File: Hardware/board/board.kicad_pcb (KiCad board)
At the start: 2 copper layers, 124 parts, among them J1 USB_C_Receptacle_USB2.0_16P, J2 Barrel_Jack_PTH, SW1 SKRPACE010, SW10 CPG151101D212, SW11 CPG151101D212, SW12 EC11E15244G1, SW13 EC11E15244G1, SW14 EC11E15244G1, SW15 EC11E15244G1, SW2 CPG151101D212, SW3 CPG151101D212, SW4 EC11E15244G1, SW5 CPG151101D212, SW6 CPG151101D212, SW7 CPG151101D212, SW8 CPG151101D212, SW9 EC11E15244G1, U1 MIC5219-3.3YM5, U10 WS2812B, U11 WS2812B, U12 WS2812B, U13 WS2812B, U14 WS2812B, U15 WS2812B, U16 WS2812B, U17 WS2812B, U18 WS2812B, U19 WS2812B, U2 MIC5219-3.3YM5, U20 WS2812B, U21 WS2812B, U22 WS2812B, U23 WS2812B, U24 WS2812B, U25 WS2812B, U26 WS2812B, U27 WS2812B, U28 WS2812B, U29 WS2812B, U3 STM32F407VETx, U30 WS2812B, U31 WS2812B, U32 WS2812B, U33 WS2812B, U34 WS2812B, U35 WS2812B, U36 WS2812B, U37 WS2812B, U38 WS2812B, U39 WS2812B, U4 PT4103B23F, U40 WS2812B, U41 WS2812B, U42 WS2812B, U43 WS2812B, U44 WS2812B, U45 WS2812B, U46 WS2812B, U47 WS2812B, U48 TPS562200DDCR, U49 TPS568215RNNR, U5 HC-FPC-0.5-40P-FH20, U50 CYA0630-4.7UH, U6 WS2812B, U7 WS2812B, U8 WS2812B, U9 WS2812B, X1 CSTNE8M00G550000R0

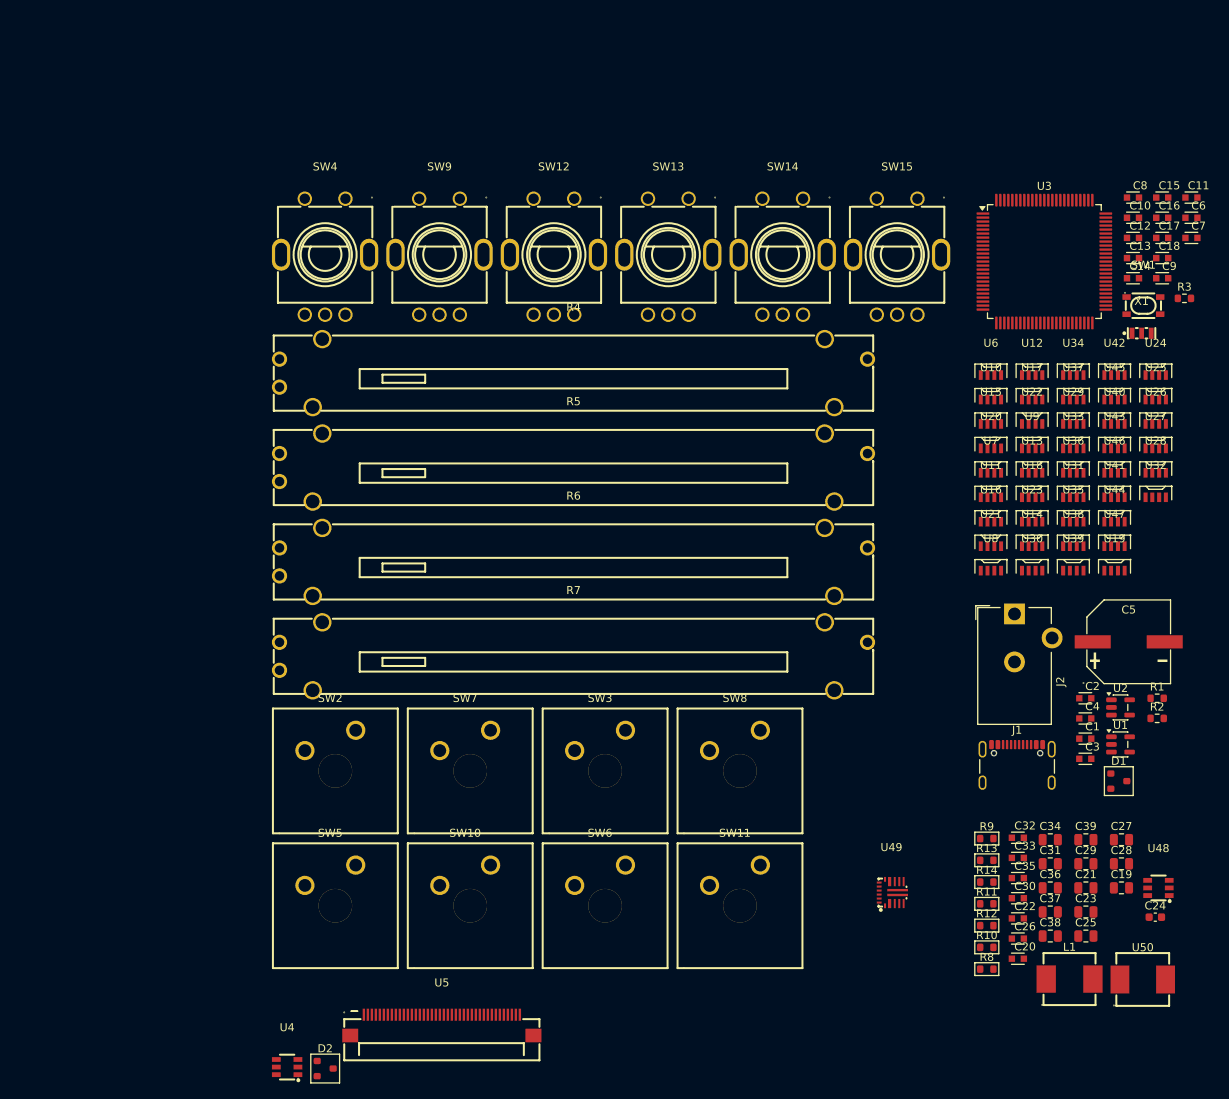
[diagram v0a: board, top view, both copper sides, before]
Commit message: sdadsa
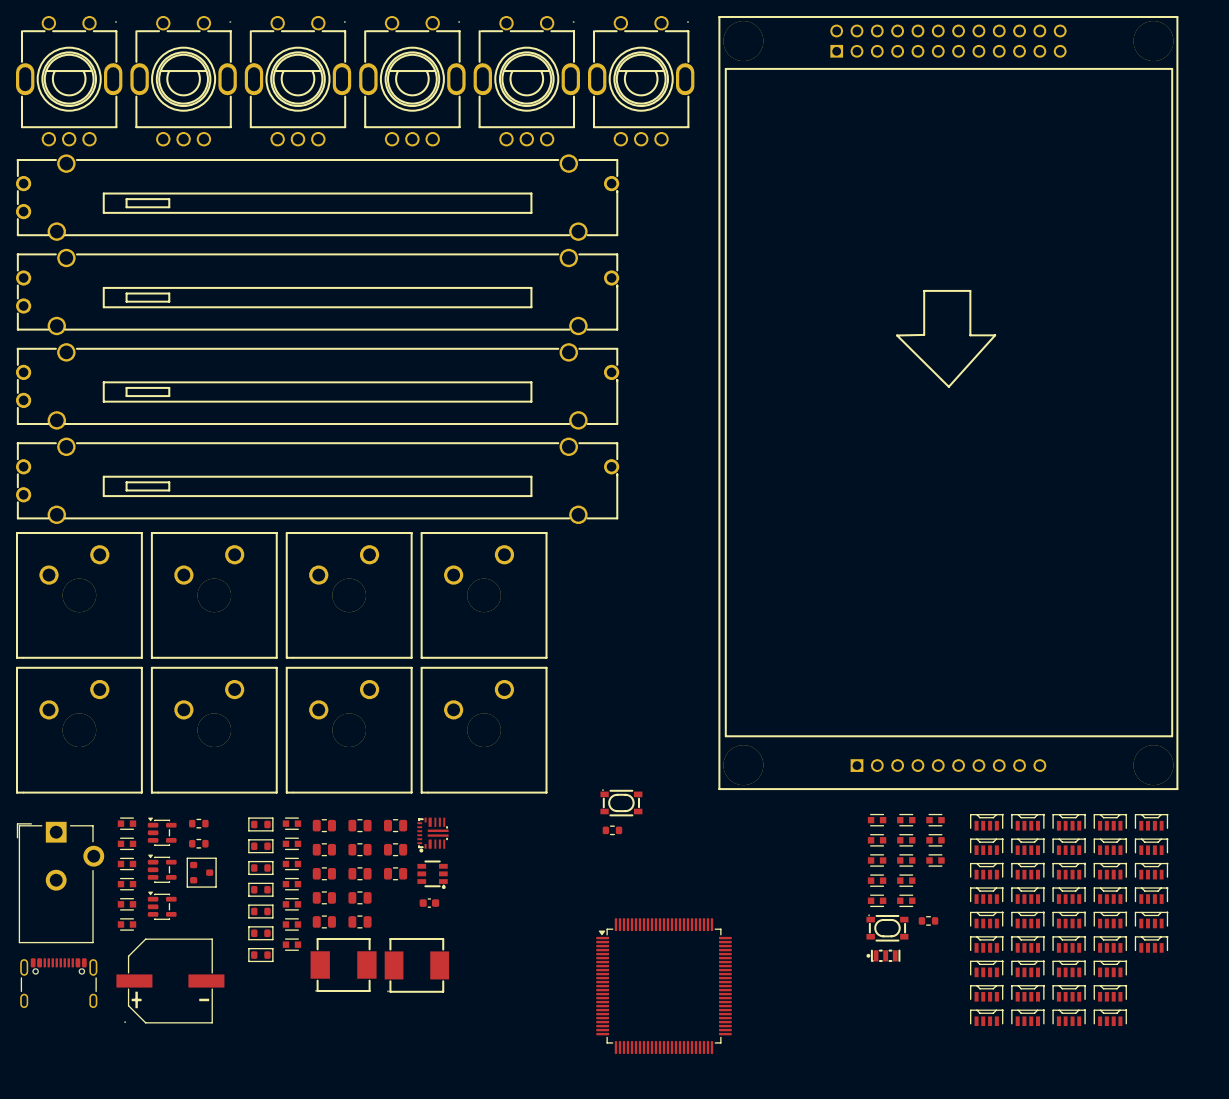
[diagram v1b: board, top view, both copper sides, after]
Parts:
- removed D2: PMEG4005CT, PCM_Package_TO_SOT_SMD_AKL:SOT-23
- removed U5: HC-FPC-0.5-40P-FH20, easyeda_imports:FPC-SMD_40P-P0.50_HC-FPC-0.5-40P-FH20
- added C40: 1uF, PCM_fab:C_0603, F.Cu at (75.3, 157.7)
- added C41: 1uF, PCM_fab:C_0603, F.Cu at (75.3, 160.2)
- added R15: 10k, Resistor_SMD:R_0603_1608Metric, F.Cu at (136.0, 148.5)
- added SW16: SKRPACE010, easyeda_imports:KEY-SMD_4P-L4.2-W3.2-P2.20-LS4.6, F.Cu at (137.1, 145.1)
- added U51: MIC5219-3.3YM5, Package_TO_SOT_SMD:SOT-23-5, F.Cu at (79.7, 158.0)
- U4: value PT4103B23F -> HS35B01A; footprint easyeda_imports:SOT-23-6_L2.9-W1.6-P0.95-LS2.8-BR -> easyeda_imports:LCD-TH_L96.5-W57.3_HS35B01A
- moved C5 127.1 mm to (80.7, 167.3)
- moved J2 122.9 mm to (66.5, 148.7)
- moved J1 122.9 mm to (66.8, 168.7)
- moved C4 121.6 mm to (75.3, 155.2)
- moved U2 121.5 mm to (79.7, 153.4)
- moved C2 121.2 mm to (75.3, 150.2)
- moved R1 120.8 mm to (84.3, 147.6)
- moved R2 120.8 mm to (84.3, 150.1)
- moved C3 120.5 mm to (75.3, 152.7)
- moved U1 120.3 mm to (79.7, 148.8)
- moved C1 120.3 mm to (75.3, 147.6)
- moved U4 117.6 mm to (178.0, 94.5)
- moved D1 115.2 mm to (84.6, 153.8)
- moved U3 102.3 mm to (142.4, 167.9)
- moved C27 100.2 mm to (100.0, 159.9)
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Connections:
- R4 pad 1: unconnected-(R4-Pad1) -> /button-encoder/+3.3V_ANALOG
- R4 pad 3: unconnected-(R4-Pad3) -> GND
- R5 pad 1: unconnected-(R5-Pad1) -> /button-encoder/+3.3V_ANALOG
- R5 pad 3: unconnected-(R5-Pad3) -> GND
- R6 pad 1: unconnected-(R6-Pad1) -> /button-encoder/+3.3V_ANALOG
- R6 pad 3: unconnected-(R6-Pad3) -> GND
- R7 pad 1: unconnected-(R7-Pad1) -> /button-encoder/+3.3V_ANALOG
- R7 pad 3: unconnected-(R7-Pad3) -> GND
- U3 pad 14: unconnected-(U3-NRST-Pad14) -> Net-(U3-NRST)
- U3 pad 21: unconnected-(U3-VREF+-Pad21) -> /mcu/+3.3V_DIGITAL
- U3 pad 94: unconnected-(U3-BOOT0-Pad94) -> /mcu/BOOT0
- U4 pad 1: unconnected-(U4-SW-Pad1) -> /display/FSMC_NE1
- U4 pad 2: GND -> /display/FSMC_A16
- U4 pad 3: unconnected-(U4-FB-Pad3) -> /display/FSMC_NWE
- U4 pad 4: /display/+3.3V_DIGITAL -> /display/FSMC_NOE
- U4 pad 5: unconnected-(U4-OV-Pad5) -> /display/LCD_RST
- U4 pad 6: /display/+5V_SYS -> /display/FSMC_D0

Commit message: holy larp is that you
holy larp is that you
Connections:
- net /bec/EN renamed EN
- net /button-encoder/FADER_1 renamed FADER_1
- net /button-encoder/FADER_2 renamed FADER_2
- net /button-encoder/FADER_3 renamed FADER_3
- net /button-encoder/FADER_4 renamed FADER_4
- net /display/BACKLIGHT_PWM renamed BACKLIGHT_PWM
- net /mcu/BOOT0 renamed BOOT0
- net /mcu/FSMC_D12 renamed FSMC_D12
- net /mcu/LED_ENC6_DATA renamed LED_ENC6_DATA
- net /mcu/SWCLK renamed SWCLK
- net /mcu/SWDIO renamed SWDIO
- net /power-usb/5V_USB renamed 5V_USB
- net /power-usb/CC1 renamed CC1
- net /power-usb/CC2 renamed CC2
- C1 pad 1: /power-usb/+5V_SYS -> +5V_SYS
- C10 pad 1: /mcu/+3.3V_DIGITAL -> +3.3V_DIGITAL
- C11 pad 1: /mcu/+3.3V_DIGITAL -> +3.3V_DIGITAL
- C12 pad 1: /mcu/+3.3V_DIGITAL -> +3.3V_DIGITAL
- C13 pad 1: /mcu/+3.3V_DIGITAL -> +3.3V_DIGITAL
- C14 pad 1: /mcu/+3.3V_DIGITAL -> +3.3V_DIGITAL
- C15 pad 1: /mcu/+3.3V_DIGITAL -> +3.3V_DIGITAL
- C16 pad 1: /mcu/+3.3V_DIGITAL -> +3.3V_DIGITAL
- C17 pad 1: /mcu/+3.3V_DIGITAL -> +3.3V_DIGITAL
- C18 pad 1: /mcu/+3.3V_DIGITAL -> +3.3V_DIGITAL
- C19 pad 2: /bec/+12V -> +12V
- C2 pad 1: /power-usb/+5V_SYS -> +5V_SYS
- C20 pad 1: /bec/+12V -> +12V
- C21 pad 2: /bec/+12V -> +12V
- C22 pad 1: /bec/+12V -> +12V
- C23 pad 2: /bec/+12V -> +12V
- C25 pad 2: /bec/+12V -> +12V
- C26 pad 1: /bec/+12V -> +12V
- C27 pad 2: /bec/+12V -> +12V
- C28 pad 2: /bec/+12V -> +12V
- C3 pad 1: /power-usb/+3.3V_DIGITAL -> +3.3V_DIGITAL
- C32 pad 1: /bec/+5V_SYS -> +5V_SYS
- C33 pad 1: /bec/+5V_SYS -> +5V_SYS
- C35 pad 1: /bec/+5V_SYS -> +5V_SYS
- C36 pad 2: /bec/+5V_LED -> +5V_LED
- C37 pad 2: /bec/+5V_LED -> +5V_LED
- C38 pad 2: /bec/+5V_LED -> +5V_LED
- C39 pad 2: /bec/+5V_LED -> +5V_LED
- C4 pad 1: /power-usb/+3.3V_DIGITAL -> +3.3V_DIGITAL
- C40 pad 1: /power-usb/+5V_SYS -> +5V_SYS
- C41 pad 1: /power-usb/+3.3V_ANALOG -> +3.3V_ANALOG
- C5 pad 1: /power-usb/+12V -> +12V
- C8 pad 1: /mcu/+3.3V_DIGITAL -> +3.3V_DIGITAL
- C9 pad 1: /mcu/+3.3V_DIGITAL -> +3.3V_DIGITAL
- D1 pad 2: /power-usb/+5V_SYS -> +5V_SYS
- D1 pad 3: /power-usb/+5V_SYS -> +5V_SYS
- J1 pad A6: /power-usb/USB_D+ -> USB_D+
- J1 pad A7: /power-usb/USB_D- -> USB_D-
- J1 pad B6: /power-usb/USB_D+ -> USB_D+
- J1 pad B7: /power-usb/USB_D- -> USB_D-
- J2 pad 1: /power-usb/+12V -> +12V
- L1 pad 2: /bec/+5V_LED -> +5V_LED
- R13 pad 2: /bec/+5V_SYS -> +5V_SYS
- R15 pad 2: /mcu/+3.3V_DIGITAL -> +3.3V_DIGITAL
- R4 pad 1: /button-encoder/+3.3V_ANALOG -> +3.3V_ANALOG
- R5 pad 1: /button-encoder/+3.3V_ANALOG -> +3.3V_ANALOG
- R6 pad 1: /button-encoder/+3.3V_ANALOG -> +3.3V_ANALOG
- R7 pad 1: /button-encoder/+3.3V_ANALOG -> +3.3V_ANALOG
- SW1 pad 3: /mcu/+3.3V_DIGITAL -> +3.3V_DIGITAL
- SW1 pad 4: /mcu/+3.3V_DIGITAL -> +3.3V_DIGITAL
- SW10 pad 1: /button-encoder/SW_7 -> SW_7
- SW11 pad 1: /button-encoder/SW_8 -> SW_8
- SW12 pad A: /button-encoder/ENC3_A -> ENC3_A
- SW12 pad B: /button-encoder/ENC3_B -> ENC3_B
- SW12 pad E: /button-encoder/ENC3_SW -> ENC3_SW
- SW13 pad A: /button-encoder/ENC4_A -> ENC4_A
- SW13 pad B: /button-encoder/ENC4_B -> ENC4_B
- SW13 pad E: /button-encoder/ENC4_SW -> ENC4_SW
- SW14 pad A: /button-encoder/ENC5_A -> ENC5_A
- SW14 pad B: /button-encoder/ENC5_B -> ENC5_B
- SW14 pad E: /button-encoder/ENC5_SW -> ENC5_SW
- SW15 pad A: /button-encoder/ENC6_A -> ENC6_A
- SW15 pad B: /button-encoder/ENC6_B -> ENC6_B
- SW15 pad E: /button-encoder/ENC6_SW -> ENC6_SW
- SW2 pad 1: /button-encoder/SW_1 -> SW_1
- SW3 pad 1: /button-encoder/SW_2 -> SW_2
- SW4 pad A: /button-encoder/ENC1_A -> ENC1_A
- SW4 pad B: /button-encoder/ENC1_B -> ENC1_B
- SW4 pad E: /button-encoder/ENC1_SW -> ENC1_SW
- SW5 pad 1: /button-encoder/SW_3 -> SW_3
- SW6 pad 1: /button-encoder/SW_4 -> SW_4
- SW7 pad 1: /button-encoder/SW_5 -> SW_5
- SW8 pad 1: /button-encoder/SW_6 -> SW_6
- SW9 pad A: /button-encoder/ENC2_A -> ENC2_A
- SW9 pad B: /button-encoder/ENC2_B -> ENC2_B
- SW9 pad E: /button-encoder/ENC2_SW -> ENC2_SW
- U1 pad 1: /power-usb/+5V_SYS -> +5V_SYS
- U1 pad 3: /power-usb/+5V_SYS -> +5V_SYS
- U1 pad 5: /power-usb/+3.3V_DIGITAL -> +3.3V_DIGITAL
- U10 pad 2: /led/+5V_LED -> +5V_LED
- U11 pad 2: /led/+5V_LED -> +5V_LED
- U12 pad 2: /led/+5V_LED -> +5V_LED
- U13 pad 2: /led/+5V_LED -> +5V_LED
- U14 pad 1: /led/LED_KEYS_DATA -> LED_KEYS_DATA
- U15 pad 2: /led/+5V_LED -> +5V_LED
- U16 pad 2: /led/+5V_LED -> +5V_LED
- U17 pad 2: /led/+5V_LED -> +5V_LED
- U18 pad 2: /led/+5V_LED -> +5V_LED
- U2 pad 1: /power-usb/+5V_SYS -> +5V_SYS
- U2 pad 3: /power-usb/+5V_SYS -> +5V_SYS
- U2 pad 5: /power-usb/+3.3V_DIGITAL -> +3.3V_DIGITAL
- U20 pad 2: /led/+5V_LED -> +5V_LED
- U21 pad 2: /led/+5V_LED -> +5V_LED
- U22 pad 2: /led/+5V_LED -> +5V_LED
- U23 pad 2: /led/+5V_LED -> +5V_LED
- U29 pad 1: /led/LED_ENC2_DATA -> LED_ENC2_DATA
- U29 pad 2: /led/+5V_LED -> +5V_LED
- U3 pad 1: /mcu/ENC4_SW -> ENC4_SW
- U3 pad 100: /mcu/+3.3V_DIGITAL -> +3.3V_DIGITAL
- U3 pad 11: /mcu/+3.3V_DIGITAL -> +3.3V_DIGITAL
- U3 pad 15: /mcu/SW_1 -> SW_1
- U3 pad 16: /mcu/SW_2 -> SW_2
- U3 pad 17: /mcu/SW_3 -> SW_3
- U3 pad 18: /mcu/SW_4 -> SW_4
- U3 pad 19: /mcu/+3.3V_DIGITAL -> +3.3V_DIGITAL
- U3 pad 2: /mcu/ENC5_A -> ENC5_A
- U3 pad 21: /mcu/+3.3V_DIGITAL -> +3.3V_DIGITAL
- U3 pad 22: /mcu/+3.3V_DIGITAL -> +3.3V_DIGITAL
- U3 pad 28: /mcu/+3.3V_DIGITAL -> +3.3V_DIGITAL
- U3 pad 3: /mcu/ENC5_B -> ENC5_B
- U3 pad 33: /mcu/SW_5 -> SW_5
- U3 pad 34: /mcu/LCD_RST -> LCD_RST
- U3 pad 35: /mcu/ENC1_A -> ENC1_A
- U3 pad 36: /mcu/ENC1_B -> ENC1_B
- U3 pad 37: /mcu/ENC1_SW -> ENC1_SW
- U3 pad 38: /mcu/FSMC_D4 -> FSMC_D4
- U3 pad 39: /mcu/FSMC_D5 -> FSMC_D5
- U3 pad 4: /mcu/ENC5_SW -> ENC5_SW
- U3 pad 40: /mcu/FSMC_D6 -> FSMC_D6
- U3 pad 41: /mcu/FSMC_D7 -> FSMC_D7
- U3 pad 42: /mcu/FSMC_D8 -> FSMC_D8
- U3 pad 43: /mcu/FSMC_D9 -> FSMC_D9
- U3 pad 44: /mcu/FSMC_D10 -> FSMC_D10
- U3 pad 45: /mcu/FSMC_D11 -> FSMC_D11
- U3 pad 47: /mcu/LED_FADER1_DATA -> LED_FADER1_DATA
- U3 pad 48: /mcu/LED_FADER2_DATA -> LED_FADER2_DATA
- U3 pad 50: /mcu/+3.3V_DIGITAL -> +3.3V_DIGITAL
- U3 pad 51: /mcu/LED_FADER3_DATA -> LED_FADER3_DATA
- U3 pad 52: /mcu/LED_FADER4_DATA -> LED_FADER4_DATA
- U3 pad 55: /mcu/FSMC_D13 -> FSMC_D13
- U3 pad 56: /mcu/FSMC_D14 -> FSMC_D14
- U3 pad 57: /mcu/FSMC_D15 -> FSMC_D15
- U3 pad 58: /mcu/FSMC_A16 -> FSMC_A16
- U3 pad 59: /mcu/LED_ENC4_DATA -> LED_ENC4_DATA
- U3 pad 6: /mcu/+3.3V_DIGITAL -> +3.3V_DIGITAL
- U3 pad 60: /mcu/LED_ENC5_DATA -> LED_ENC5_DATA
- U3 pad 61: /mcu/FSMC_D0 -> FSMC_D0
- U3 pad 62: /mcu/FSMC_D1 -> FSMC_D1
- U3 pad 63: /mcu/SW_6 -> SW_6
- U3 pad 64: /mcu/SW_7 -> SW_7
- U3 pad 65: /mcu/ENC6_A -> ENC6_A
- U3 pad 66: /mcu/ENC6_B -> ENC6_B
- U3 pad 67: /mcu/LED_KEYS_DATA -> LED_KEYS_DATA
- U3 pad 70: /mcu/USB_D- -> USB_D-
- U3 pad 71: /mcu/USB_D+ -> USB_D+
- U3 pad 75: /mcu/+3.3V_DIGITAL -> +3.3V_DIGITAL
- U3 pad 78: /mcu/ENC6_SW -> ENC6_SW
- U3 pad 79: /mcu/SW_8 -> SW_8
- U3 pad 81: /mcu/FSMC_D2 -> FSMC_D2
- U3 pad 82: /mcu/FSMC_D3 -> FSMC_D3
- U3 pad 83: /mcu/LED_ENC1_DATA -> LED_ENC1_DATA
- U3 pad 84: /mcu/LED_ENC2_DATA -> LED_ENC2_DATA
- U3 pad 85: /mcu/FSMC_NOE -> FSMC_NOE
- U3 pad 86: /mcu/FSMC_NWE -> FSMC_NWE
- U3 pad 87: /mcu/LED_ENC3_DATA -> LED_ENC3_DATA
- U3 pad 88: /mcu/FSMC_NE1 -> FSMC_NE1
- U3 pad 90: /mcu/ENC2_A -> ENC2_A
- U3 pad 91: /mcu/ENC2_B -> ENC2_B
- U3 pad 92: /mcu/ENC2_SW -> ENC2_SW
- U3 pad 93: /mcu/ENC3_A -> ENC3_A
- U3 pad 95: /mcu/ENC3_B -> ENC3_B
- U3 pad 96: /mcu/ENC3_SW -> ENC3_SW
- U3 pad 97: /mcu/ENC4_A -> ENC4_A
- U3 pad 98: /mcu/ENC4_B -> ENC4_B
- U30 pad 1: /led/LED_ENC1_DATA -> LED_ENC1_DATA
- U30 pad 2: /led/+5V_LED -> +5V_LED
- U31 pad 1: /led/LED_ENC3_DATA -> LED_ENC3_DATA
- U31 pad 2: /led/+5V_LED -> +5V_LED
- U33 pad 2: /led/+5V_LED -> +5V_LED
- U34 pad 2: /led/+5V_LED -> +5V_LED
- U35 pad 2: /led/+5V_LED -> +5V_LED
- U36 pad 2: /led/+5V_LED -> +5V_LED
- U37 pad 2: /led/+5V_LED -> +5V_LED
- U38 pad 2: /led/+5V_LED -> +5V_LED
- U39 pad 1: /led/LED_ENC3_DATA -> LED_ENC3_DATA
- U39 pad 2: /led/+5V_LED -> +5V_LED
- U4 pad 1: /display/FSMC_NE1 -> FSMC_NE1
- U4 pad 10: /display/FSMC_D4 -> FSMC_D4
- U4 pad 11: /display/FSMC_D5 -> FSMC_D5
- U4 pad 12: /display/FSMC_D6 -> FSMC_D6
- U4 pad 13: /display/FSMC_D7 -> FSMC_D7
- U4 pad 14: /display/FSMC_D8 -> FSMC_D8
- U4 pad 15: /display/FSMC_D9 -> FSMC_D9
- U4 pad 16: /display/FSMC_D10 -> FSMC_D10
- U4 pad 17: /display/FSMC_D11 -> FSMC_D11
- U4 pad 19: /display/FSMC_D13 -> FSMC_D13
- U4 pad 2: /display/FSMC_A16 -> FSMC_A16
- U4 pad 20: /display/FSMC_D14 -> FSMC_D14
- U4 pad 21: /display/FSMC_D15 -> FSMC_D15
- U4 pad 26: /display/+3.3V_DIGITAL -> +3.3V_DIGITAL
- U4 pad 3: /display/FSMC_NWE -> FSMC_NWE
- U4 pad 32: /display/+3.3V_DIGITAL -> +3.3V_DIGITAL
- U4 pad 4: /display/FSMC_NOE -> FSMC_NOE
- U4 pad 5: /display/LCD_RST -> LCD_RST
- U4 pad 6: /display/FSMC_D0 -> FSMC_D0
- U4 pad 7: /display/FSMC_D1 -> FSMC_D1
- U4 pad 8: /display/FSMC_D2 -> FSMC_D2
- U4 pad 9: /display/FSMC_D3 -> FSMC_D3
- U40 pad 1: /led/LED_ENC4_DATA -> LED_ENC4_DATA
- U40 pad 2: /led/+5V_LED -> +5V_LED
- U41 pad 1: /led/LED_ENC5_DATA -> LED_ENC5_DATA
- U41 pad 2: /led/+5V_LED -> +5V_LED
- U42 pad 2: /led/+5V_LED -> +5V_LED
- U43 pad 2: /led/+5V_LED -> +5V_LED
- U44 pad 2: /led/+5V_LED -> +5V_LED
- U45 pad 2: /led/+5V_LED -> +5V_LED
- U46 pad 2: /led/+5V_LED -> +5V_LED
- U47 pad 2: /led/+5V_LED -> +5V_LED
- U48 pad 3: /bec/+12V -> +12V
- U49 pad 11: /bec/+12V -> +12V
- U49 pad 2: /bec/+12V -> +12V
- U50 pad 2: /bec/+5V_SYS -> +5V_SYS
- U51 pad 1: /power-usb/+5V_SYS -> +5V_SYS
- U51 pad 3: /power-usb/+5V_SYS -> +5V_SYS
- U51 pad 5: /power-usb/+3.3V_ANALOG -> +3.3V_ANALOG
- U6 pad 1: /led/LED_FADER1_DATA -> LED_FADER1_DATA
- U6 pad 2: /led/+5V_LED -> +5V_LED
- U7 pad 1: /led/LED_FADER2_DATA -> LED_FADER2_DATA
- U7 pad 2: /led/+5V_LED -> +5V_LED
- U8 pad 1: /led/LED_FADER3_DATA -> LED_FADER3_DATA
- U8 pad 2: /led/+5V_LED -> +5V_LED
- U9 pad 1: /led/LED_FADER4_DATA -> LED_FADER4_DATA
- U9 pad 2: /led/+5V_LED -> +5V_LED
